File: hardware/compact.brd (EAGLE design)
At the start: 98.7 x 80 mm, 57 parts, among them IC1 ATMEGA168-20P, IC2 74AC74N, IC3 MAX232, IC4 74AC74N, Q1 16MHz, T1 BF199

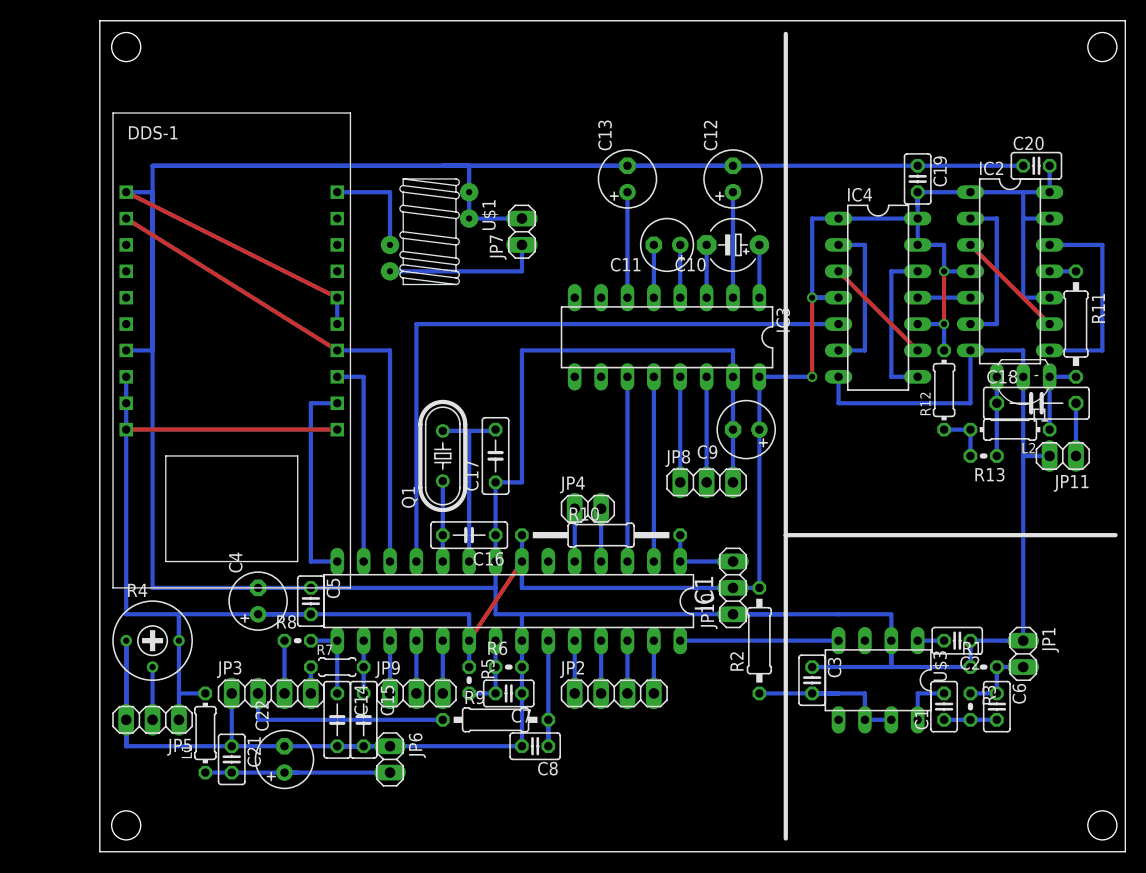
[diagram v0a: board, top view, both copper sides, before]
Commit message: Updated hardware.
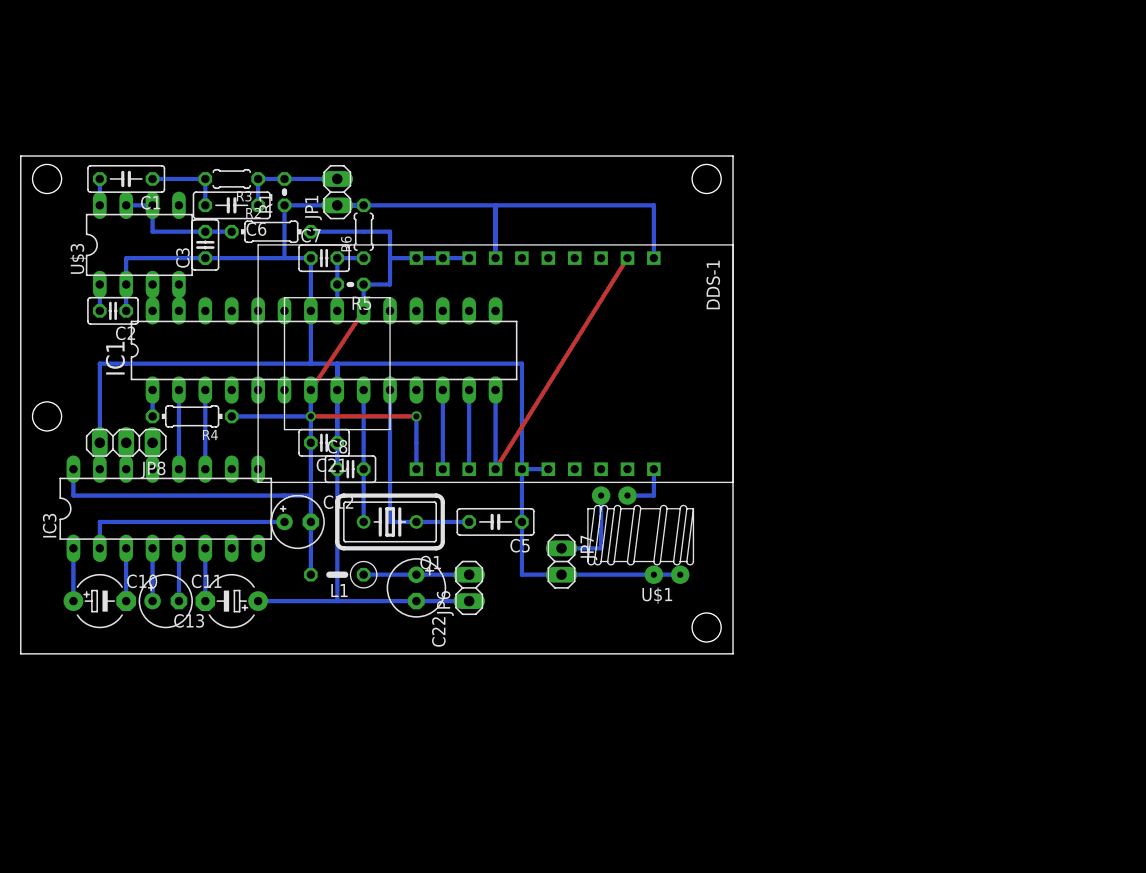
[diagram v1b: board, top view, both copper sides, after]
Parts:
- removed C14, C15: 100nF, rcl:C050-025X075
- removed C16, C17: 22pF, rcl:C050-025X075
- removed C18: 100nF, rcl:C075-032X103
- removed C19, C20: 100nF, rcl:C025-025X050
- removed C4: 100uF, rcl:E2,5-6
- removed C9: 1uF, rcl:E2,5-6
- removed IC2, IC4: 74AC74N, 74xx-eu:DIL14
- removed JP10: PRG2, pinhead:1X03
- removed JP11: F-IN, pinhead:1X02
- removed JP2: DISP DATA, pinhead:1X04
- removed JP3: ROT, pinhead:1X04
- removed JP4: DISP CTRL, pinhead:1X02
- removed JP5: DISP SUPPLY, pinhead:1X03
- removed JP9: PRG1, pinhead:1X03
- removed L2: 470uH, rcl:0204/7
- removed R10: 10k, rcl:0207/15
- removed R11: 470, rcl:0207/10
- removed R12: 470, rcl:0204/7
- removed R13, R8: 10k, rcl:0204V
- removed R7: 10k, rcl:0204/5
- removed R9: 10k, rcl:0207/10
- removed T1: BF199, transistor-neu-to92:TO92-CEB
- C1, C6: device rcl:C025-025X050 -> rcl:C050-025X075
- C12: device rcl:E2,5-6 -> rcl:E2,5-5
- C13: device rcl:E2,5-6 -> rcl:E5-5
- C5: value 100nF -> 22pF; device rcl:C025-025X050 -> rcl:C050-025X075
- C8: value 100nF -> 22pF
- IC1: value ATMEGA168-20P -> MEGA8-PU; device adafruit:DIL28-3 -> avr-6:DIL28-3
- L1: device rcl:0204/7 -> rcl:0207/5V
- Q1: device crystal:HC49/S -> crystal:HC18U-V
- R2: device rcl:0207/10 -> rcl:0204/7
- R3, R6: device rcl:0204V -> rcl:0204/5
- R4: device rcl:RTRIM3339P -> rcl:0204/7
- moved C1 93.7 mm to (7.62, 64.8), turned to 180 degrees
- moved C6 88.1 mm to (17.8, 62.2), turned to 180 degrees
- moved R3 87.4 mm to (17.8, 64.8), turned to 180 degrees
- moved C2 87.3 mm to (6.35, 52.1)
- moved U$3 82.5 mm to (8.89, 58.4), turned to 0 degrees
- moved R1 81.4 mm to (22.9, 63.5), turned to 90 degrees
- moved JP1 79.6 mm to (27.9, 63.5), turned to 90 degrees
- moved C3 71.9 mm to (15.2, 58.4), turned to 90 degrees
- moved C10 69.9 mm to (5.08, 24.1), turned to 0 degrees
- moved R2 61.3 mm to (21.6, 59.7), turned to 0 degrees
- moved C11 59.2 mm to (11.4, 24.1), turned to 0 degrees
- moved JP8 56.0 mm to (7.62, 39.4), turned to 180 degrees
- moved C13 55.7 mm to (17.8, 24.1), turned to 180 degrees
- moved C12 53.4 mm to (24.1, 31.8), turned to 0 degrees
- moved IC3 51.0 mm to (11.4, 33.0), turned to 0 degrees
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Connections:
- removed net N$20: IC1.24, JP2.1
- removed net N$21: C15.1, IC1.16, R7.2
- removed net N$23: C14.1, IC1.15, R8.2
- removed net N$24: JP3.4, R7.1
- removed net N$25: IC1.4, JP4.2
- removed net N$26: IC1.14, U$2.CLK
- removed net N$27: IC1.5, JP4.1
- removed net N$28: JP5.2, R4.2
- removed net N$30: IC1.12, U$2.D7, U$2.D7_2
- removed net N$31: JP3.3, R8.1
- removed net N$32: JP3.2, R9.1
- removed net N$33: C8.1, IC1.23, R9.2
- removed net N$36: C13.+, IC3.6
- removed net N$37: C16.2, IC1.10, Q1.1
- removed net N$42: C17.2, IC1.9, Q1.2
- removed net N$45: IC4.2, IC4.6
- removed net N$46: IC1.11, IC4.5
- removed net N$47: IC2.12, IC2.8
- removed net N$48: IC2.2, IC2.6
- removed net N$49: IC4.12, IC4.8
- removed net N$50: IC2.3, IC2.9
- removed net N$51: IC2.5, IC4.11
- removed net N$52: IC4.3, IC4.9
- removed net N$53: IC2.11, R11.1
- removed net N$54: L2.1, R11.2, T1.C
- removed net N$55: L2.2, R12.1, R13.2
- removed net N$56: C18.1, R13.1, T1.B
- removed net N$57: C18.2, JP11.1
- removed net N$7 (its old number): IC1.1, JP10.3, R10.2
- net GND: now also C13.+, C8.1; no longer C12.-, C13.-, C14.2, C15.2, C16.1, C17.1, C19.1, C20.1, C4.-, C8.2, C9.-, IC2.7, IC4.7, JP10.1, JP11.2, JP3.1, JP5.3, R4.1, T1.E
- net N$1: now also IC1.1, R4.2; no longer IC1.17, JP9.1
- net N$10: no longer C21.2
- net N$16: now also C13.-, IC3.6; no longer IC1.27, JP2.4
- net N$18: now also IC1.12, U$2.CLK; no longer IC1.26, JP2.3
- net N$19: now also IC1.14, U$2.D7, U$2.D7_2; no longer IC1.25, JP2.2
- net N$5: now also C5.2, IC1.10, Q1.1; no longer IC1.18, JP9.2
- net N$6: now also C8.2, IC1.9, Q1.2; no longer IC1.19, JP9.3
- net N$9: now also IC1.27; no longer IC1.28
- net VCC: now also C12.-, C21.2, R4.1; no longer C19.2, C20.2, C4.+, C5.2, C9.+, IC2.1, IC2.10, IC2.13, IC2.14, IC2.4, IC4.1, IC4.10, IC4.13, IC4.14, IC4.4, JP10.2, JP5.1, R10.1, R12.2, R4.3
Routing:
- net GND: track 556.1 -> 233.7 mm
- net VCC: track 254.3 -> 103.1 mm, vias 4 -> 2
- net N$46: track 63.5 -> 0.00 mm
- net N$30: track 49.4 -> 0.00 mm
- net N$19: track 5.08 -> 31.6 mm
- net N$26: track 20.3 -> 0.00 mm
- net N$47: track 20.3 -> 0.00 mm
- net N$32: track 20.3 -> 0.00 mm
- net N$42: track 20.3 -> 0.00 mm
- net N$5: track 5.08 -> 20.3 mm
- net N$49: track 15.2 -> 0.00 mm
- net N$48: track 15.2 -> 0.00 mm
- net N$45: track 15.2 -> 0.00 mm
- net N$9: track 15.2 -> 2.54 mm
- net N$33: track 12.7 -> 0.00 mm
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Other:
- board size 98.7 x 80 mm -> 68.6 x 47.9 mm

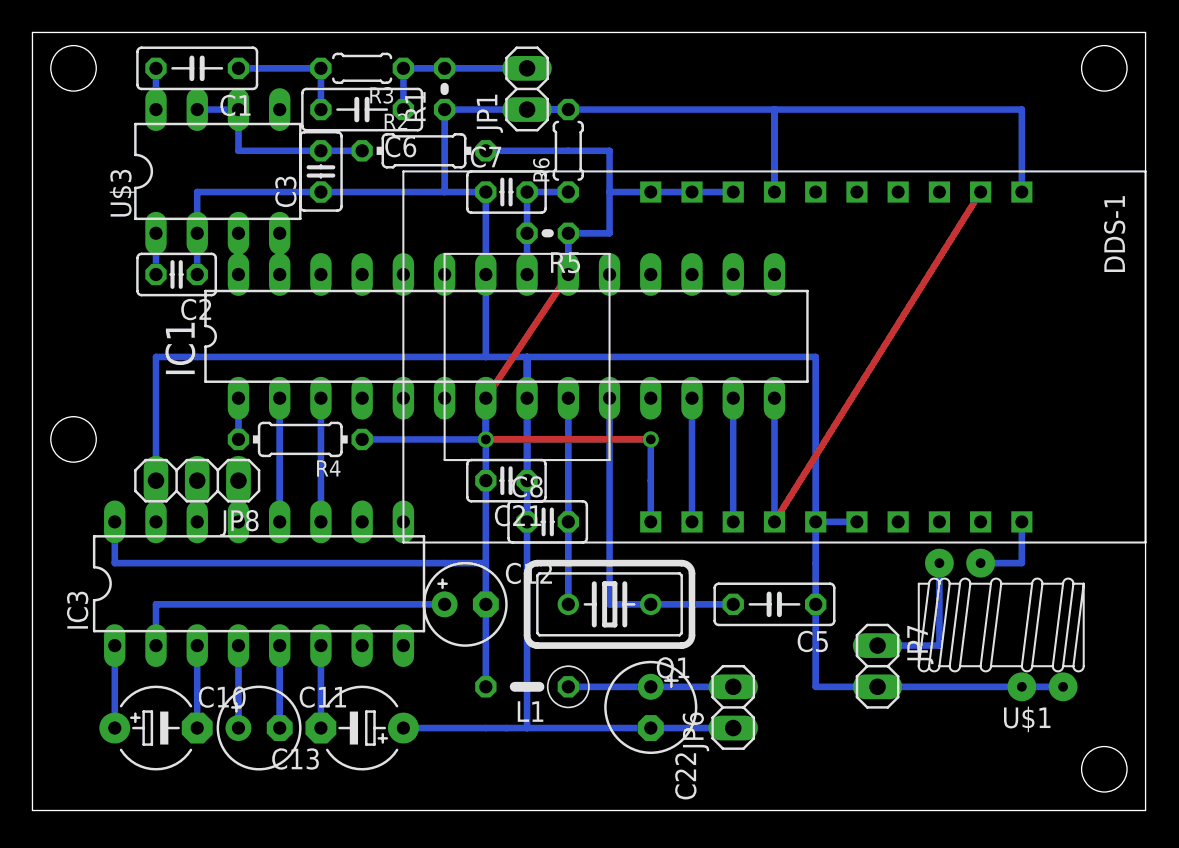
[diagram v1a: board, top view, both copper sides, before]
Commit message: Fixed circuit and board.
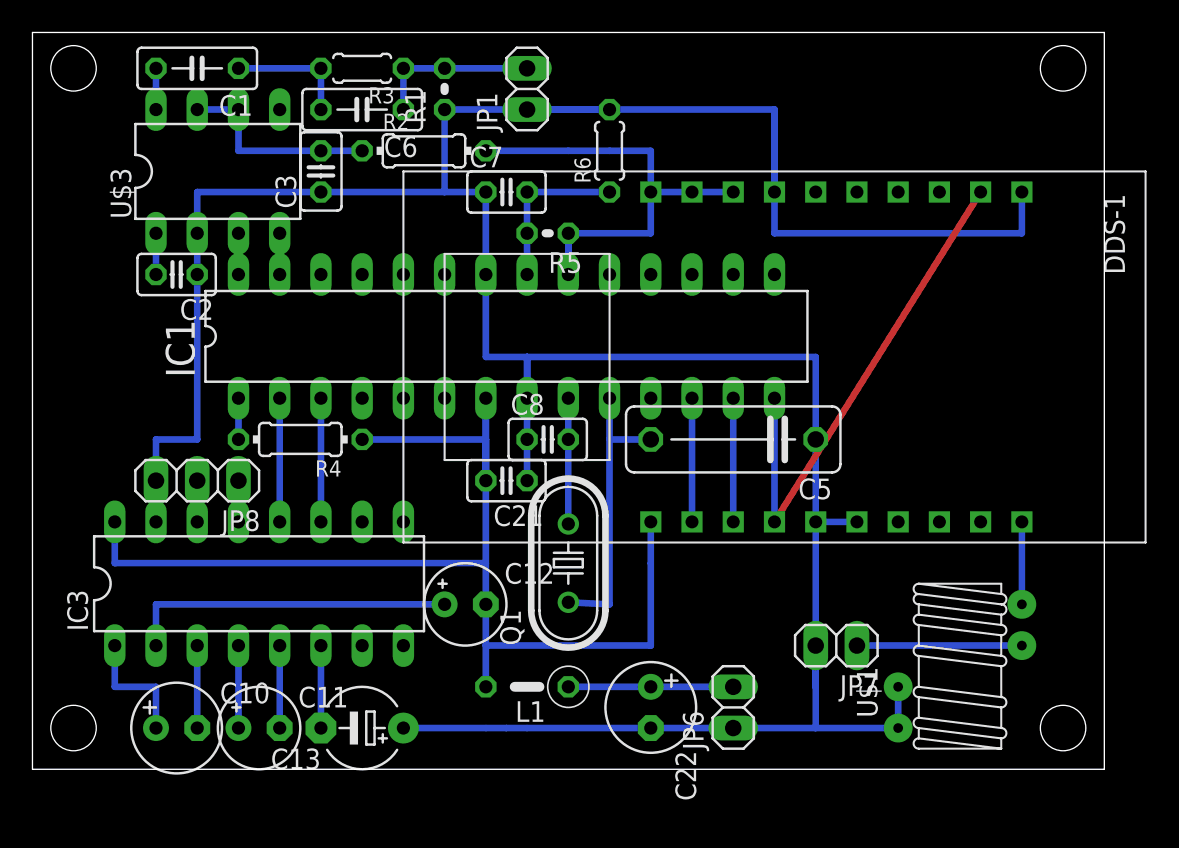
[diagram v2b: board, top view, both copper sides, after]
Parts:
- C10: device rcl:E5-5 -> rcl:E2,5-6
- C5: device rcl:C050-025X075 -> rcl:C102-043X133
- JP8: value RS-232 -> RS-232 GndTxRx
- Q1: device crystal:HC18U-V -> crystal:HC49U-V
- moved C5 10.5 mm to (40.6, 41.9)
- moved C8 5.08 mm to (29.2, 41.9)
- moved Q1 3.59 mm to (30.5, 34.3), turned to 90 degrees
- moved U$1 3.59 mm to (54.6, 27.9), turned to 0 degrees
- moved JP7 2.84 mm to (47.0, 29.2), turned to 180 degrees
- moved R6 2.54 mm to (33.0, 59.7)
- moved C10 1.27 mm to (6.35, 24.1)
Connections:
- removed net N$13: U$1.C1B, U$2.JOUT2
- new net N$1: U$1.C2B, U$2.JOUT2
- net N$14: now also U$1.C1B; no longer U$1.C2B
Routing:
- net GND: track 233.7 -> 207.0 mm
- net VCC: track 103.1 -> 109.2 mm, vias 2 -> 0
- net N$13: track 5.08 -> 0.00 mm
- net N$1: track 0.00 -> 5.08 mm
- net N$6: track 12.7 -> 7.75 mm
- net N$29: track 7.62 -> 10.2 mm
- net N$38: track 5.08 -> 7.62 mm
- net N$5: track 20.3 -> 17.8 mm
- net N$14: track 8.89 -> 10.2 mm
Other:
- board size 68.6 x 47.9 mm -> 66 x 45.4 mm

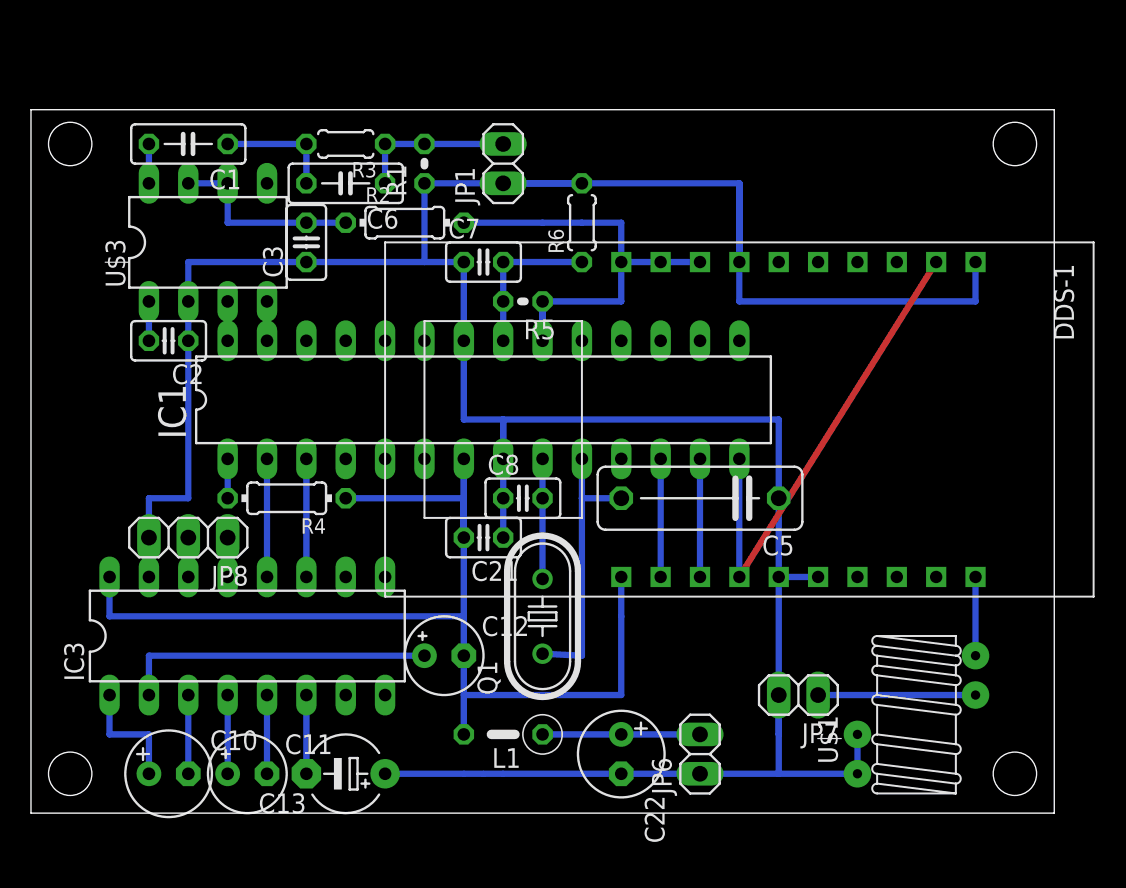
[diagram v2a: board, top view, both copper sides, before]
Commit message: Fixes.
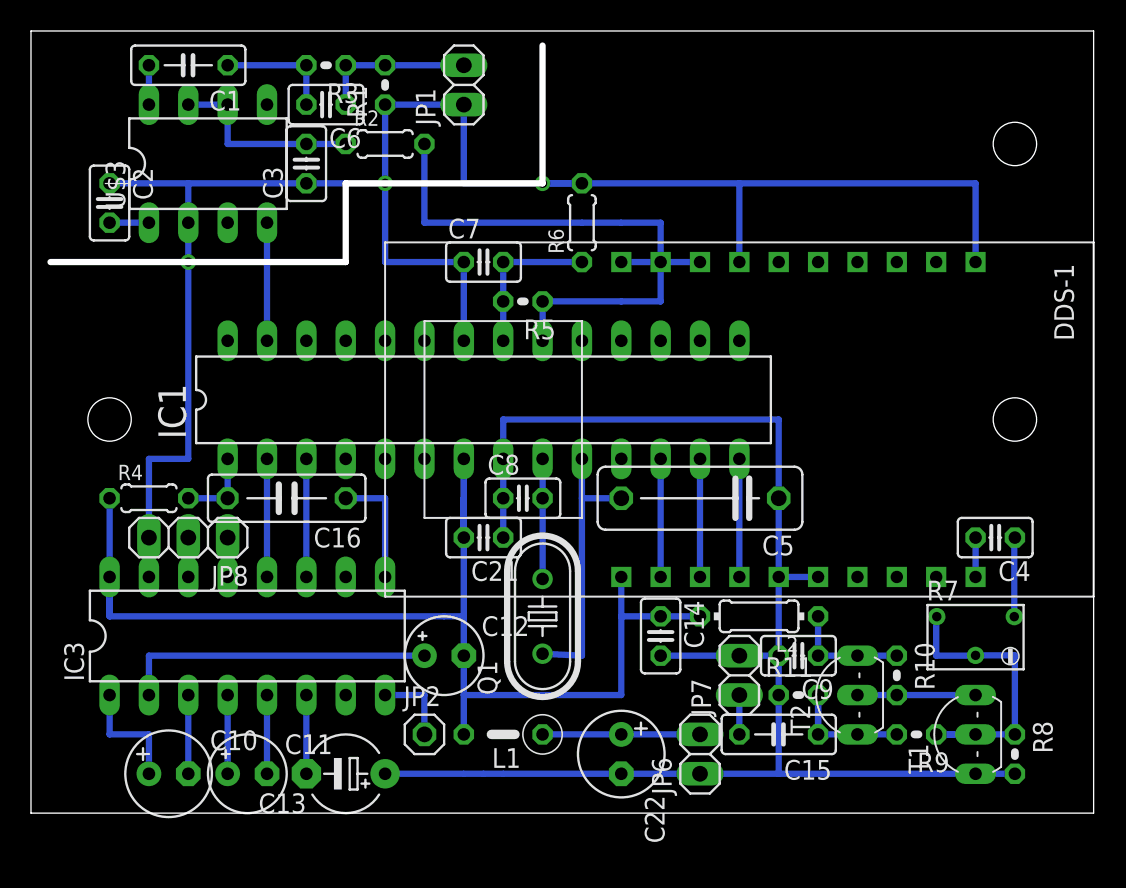
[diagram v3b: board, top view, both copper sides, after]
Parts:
- removed U$2: DDS-1, minikits:DDS-1
- added C14, C9: 220nF, rcl:C025-025X050
- added C15: 100nF, rcl:C050-025X075
- added C16: 100nF, rcl:C075-032X103
- added C4: 100nF, rcl:C025-025X050
- added JP2: DTR, pinhead:1X01
- added L2: 10uH, rcl:0204/7
- added R10, R11, R9: 220, rcl:0204V
- added R7: 1k, resistor:RTRIM74W
- added R8: 100, rcl:0204V
- added T1, T2: 2N3904, transistor-neu-to92:TO92-EBC
- C6: device rcl:C050-025X075 -> rcl:C025-025X050
- R2, R4: device rcl:0204/7 -> rcl:0204/5
- R3: device rcl:0204/5 -> rcl:0204V
- U$1: value T37_TRANSFORMER -> DDS-1; device toroid:T37_TRANSFORMER -> minikits:DDS-1
- moved U$1 22.2 mm to (45.7, 48.3), turned to 90 degrees
- moved C2 9.67 mm to (2.54, 61.0), turned to 270 degrees
- moved R4 8.89 mm to (5.08, 41.9), turned to 0 degrees
- moved JP1 5.68 mm to (25.4, 68.6)
- moved R1 5.68 mm to (20.3, 68.6)
- moved C6 5.24 mm to (16.5, 67.3)
- moved R2 5.24 mm to (20.3, 64.8)
- moved R3 5.24 mm to (16.5, 69.8)
- moved C1 5.08 mm to (7.62, 69.8)
- moved C3 5.08 mm to (15.2, 63.5)
- moved U$3 5.08 mm to (8.89, 63.5)
- moved JP7 4.02 mm to (43.2, 30.5), turned to 90 degrees
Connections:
- new net N$13: C4.1, R7.3
- new net N$20: C9.1, L2.1, R10.1, T2.C
- new net N$21: R10.2, T1.C, T2.B
- new net N$23: C15.2, JP7.1
- new net N$24: C15.1, R11.2, R9.2, T2.E
- new net N$26: C16.1, IC3.9
- new net N$27: IC3.8, JP2.1
- net GND: now also C14.2, C9.2, R11.1, R8.2, T1.E, U$1.D2, U$1.GND, U$1.GND2, U$1.RESET; no longer U$1.C1A, U$1.C2A, U$2.D2, U$2.GND, U$2.GND2, U$2.RESET
- net N$1: now also C4.2, U$1.JOUT2; no longer U$1.C2B, U$2.JOUT2
- net N$14: now also R7.1, R7.2, R8.1, R9.1, T1.B; no longer JP7.1, U$1.C1B
- net N$15: now also U$1.FQ_UP; no longer U$2.FQ_UP
- net N$18: now also U$1.CLK; no longer U$2.CLK
- net N$19: now also U$1.D7, U$1.D7_2; no longer U$2.D7, U$2.D7_2
- net N$25: now also C16.2
- net VCC: now also C14.1, L2.2, U$1.D0, U$1.D1, U$1.VCC, U$1.VCC2; no longer U$2.D0, U$2.D1, U$2.VCC, U$2.VCC2
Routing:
- net N$19: track 31.6 -> 7.62 mm
- net GND: track 207.0 -> 226.1 mm, vias 0 -> 3
- net VCC: track 109.2 -> 124.5 mm
- net N$14: track 10.2 -> 20.4 mm
- net N$24: track 0.00 -> 10.2 mm
- net N$21: track 0.00 -> 7.62 mm
- net N$20: track 0.00 -> 7.62 mm
- net N$26: track 0.00 -> 7.62 mm
- net N$13: track 0.00 -> 5.14 mm
- net N$9: track 2.54 -> 7.62 mm
- net N$27: track 0.00 -> 5.08 mm
- net N$25: track 2.54 -> 5.08 mm
- net N$23: track 0.00 -> 2.54 mm
- net N$1: track 5.08 -> 2.54 mm
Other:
- board size 66 x 45.4 mm -> 68.6 x 50.5 mm
